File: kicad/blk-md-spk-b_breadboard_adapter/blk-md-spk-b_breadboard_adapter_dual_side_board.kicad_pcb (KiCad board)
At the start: 2 copper layers, 24.1 x 29.8 mm, 12 parts, among them J1 SCJ368R1NUS0B00G, P1 CONNECTOR, P2 CONNECTOR, U1 BLK-MD-SPK-B

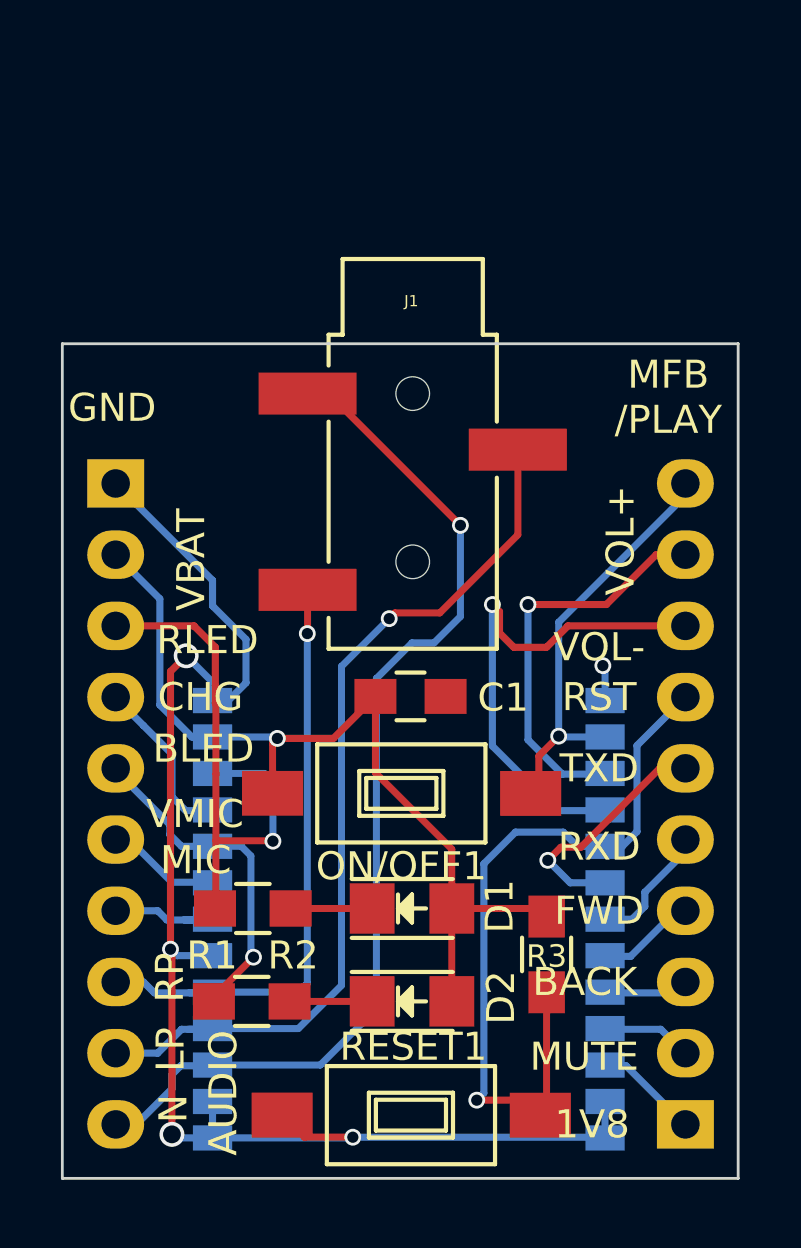
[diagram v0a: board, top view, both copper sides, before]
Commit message: updated version
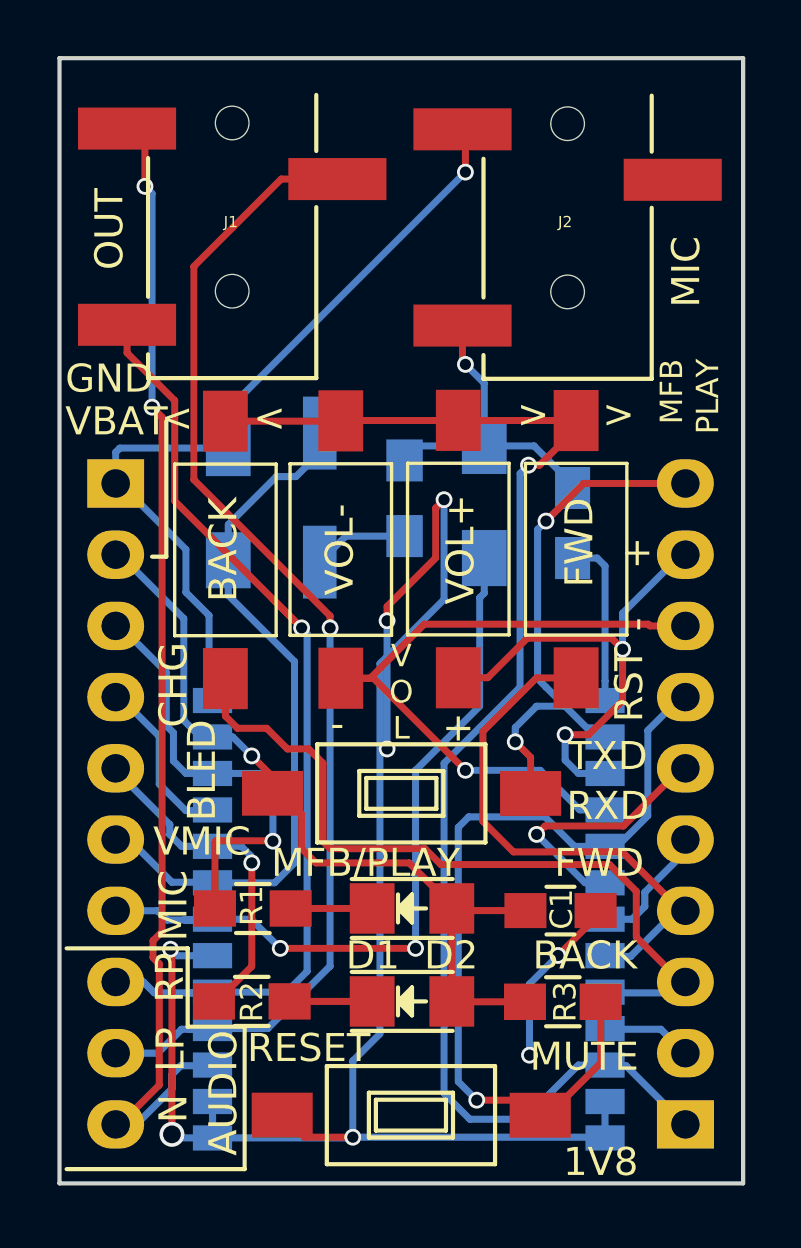
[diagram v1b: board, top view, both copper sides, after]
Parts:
- added BACK: SW_PUSH, Buttons_Switches_SMD:SW_SPST_FSMSM, F.Cu at (115.6, 108.2)
- added C2: 4u7, Capacitors_SMD:C_1206_HandSoldering, B.Cu at (115.7, 106.6)
- added C3: 1u, Capacitors_SMD:C_1206_HandSoldering, B.Cu at (124.9, 106.5)
- added C4: 10, Capacitors_SMD:C_0805_HandSoldering, B.Cu at (128.0, 107.3)
- added FWD: SW_PUSH, Buttons_Switches_SMD:SW_SPST_FSMSM, F.Cu at (128.2, 108.2)
- added J2: Jack_3.5mm_3pin, jacks:3.5mm_stereo_jack_PJ320B, F.Cu at (127.9, 93.0)
- added L1: 15n, Choke_SMD.pretty:Choke_SMD_1206_Handsoldering, B.Cu at (119.0, 106.4)
- added R4: 2k7, Resistors_SMD:R_0805_HandSoldering, B.Cu at (122.0, 106.4)
- added VOL+: SW_PUSH, Buttons_Switches_SMD:SW_SPST_FSMSM, F.Cu at (124.0, 108.2)
- added VOL-: SW_PUSH, Buttons_Switches_SMD:SW_SPST_FSMSM, F.Cu at (119.8, 108.2)
- J1: value SCJ368R1NUS0B00G -> Jack_3.5mm_3pin
- moved J1 11.6 mm to (115.9, 93.0)
- moved C1 9.33 mm to (127.6, 121.1), turned to 180 degrees
- moved R3 1.79 mm to (127.7, 124.3), turned to 180 degrees
- renumbered ON/OFF1 to MFB/PLAY, RESET1 to RESET
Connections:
- net Net-(J1-Pad1) renamed /SPKN
- net Net-(ON/OFF1-Pad1) renamed /MFB
- net Net-(P1-Pad1) renamed /1V8
- net Net-(P1-Pad2) renamed /MUTE
- net Net-(P1-Pad3) renamed /BACK
- net Net-(P1-Pad4) renamed /FWD
- net Net-(P1-Pad5) renamed /RXD
- net Net-(P1-Pad6) renamed /TXD
- net Net-(P1-Pad7) renamed /RST
- net Net-(P1-Pad8) renamed /VOL-
- net Net-(P1-Pad9) renamed /VOL+
- net Net-(P2-Pad3) renamed /RLED
- net Net-(P2-Pad4) renamed /CHG
- net Net-(P2-Pad5) renamed /BLED
- net Net-(P2-Pad6) renamed /VMIC
- net Net-(P2-Pad7) renamed /MIC
- C1 pad 1: Net-(C1-Pad1) -> GND
- C1 pad 2: GND -> /VBAT
- D1 pad 2: Net-(C1-Pad1) -> /VBAT
- D2 pad 2: Net-(C1-Pad1) -> /VBAT
- J1 pad 2: Net-(J1-Pad2) -> /SPKRP
- MFB/PLAY pad 2: Net-(C1-Pad1) -> /VBAT
- P2 pad 2: Net-(C1-Pad1) -> /VBAT
- P2 pad 8: Net-(J1-Pad4) -> /SPKRP
- P2 pad 9: Net-(J1-Pad2) -> /SPKLP
- R3 pad 2: Net-(C1-Pad1) -> /VBAT
- U1 pad 12: Net-(C1-Pad1) -> /VBAT
- U1 pad 4: Net-(J1-Pad2) -> /SPKLP
- U1 pad 5: Net-(J1-Pad4) -> /SPKRP
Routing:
- net GND: track 53.6 -> 105.1 mm, vias 5 -> 9
- net /1V8: track 3.88 -> 49.5 mm, vias 0 -> 1
- net /SPKLP: track 0.00 -> 42.8 mm, vias 0 -> 1
- net /SPKRP: track 0.00 -> 35.1 mm, vias 0 -> 1
- net Net-(C1-Pad1): track 33.1 -> 0.00 mm, vias 1 -> 0
- net Net-(J1-Pad2): track 32.2 -> 0.00 mm, vias 1 -> 0
- net /VBAT: track 0.00 -> 29.8 mm, vias 0 -> 1
- net /BACK: track 3.18 -> 28.1 mm
- net /MIC: track 4.27 -> 26.9 mm, vias 0 -> 2
- net Net-(J1-Pad4): track 21.8 -> 0.00 mm, vias 1 -> 0
- net /VMIC: track 3.95 -> 25.2 mm
- net /FWD: track 3.69 -> 19.6 mm
- net Net-(C3-Pad1): track 0.00 -> 11.5 mm, vias 0 -> 1
- net /VOL-: track 18.1 -> 24.5 mm
- net /MFB: track 15.0 -> 19.7 mm, vias 1 -> 2
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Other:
- board size 24.1 x 29.8 mm -> 24.4 x 40.1 mm
- board text added: "+"
- board text added: "-"
- board text added: "<"
- board text added: ">"
- board text added: "MFB PLAY"
- board text added: "OUT"
- board text added: "V O L"
- board text removed: "MFB /PLAY"
- board text removed: "RLED"
- board text removed: "VOL+"
- board text removed: "VOL-"
